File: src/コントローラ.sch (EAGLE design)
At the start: 13 parts, among them SW1 TOGGLESWITCH

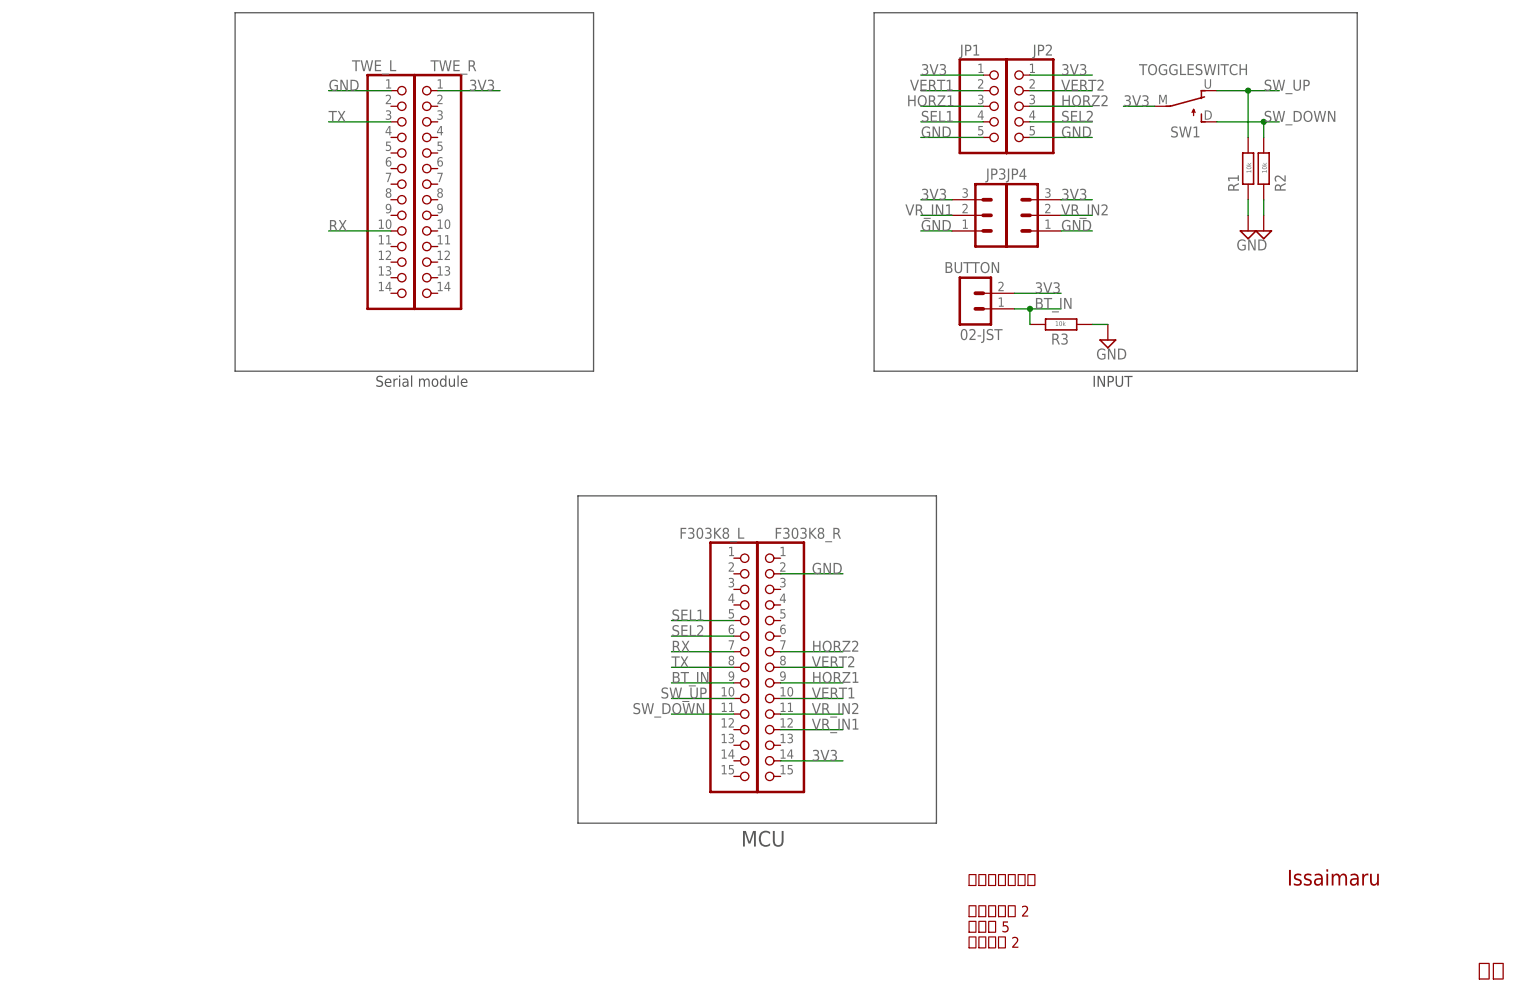
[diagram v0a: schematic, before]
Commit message: fix
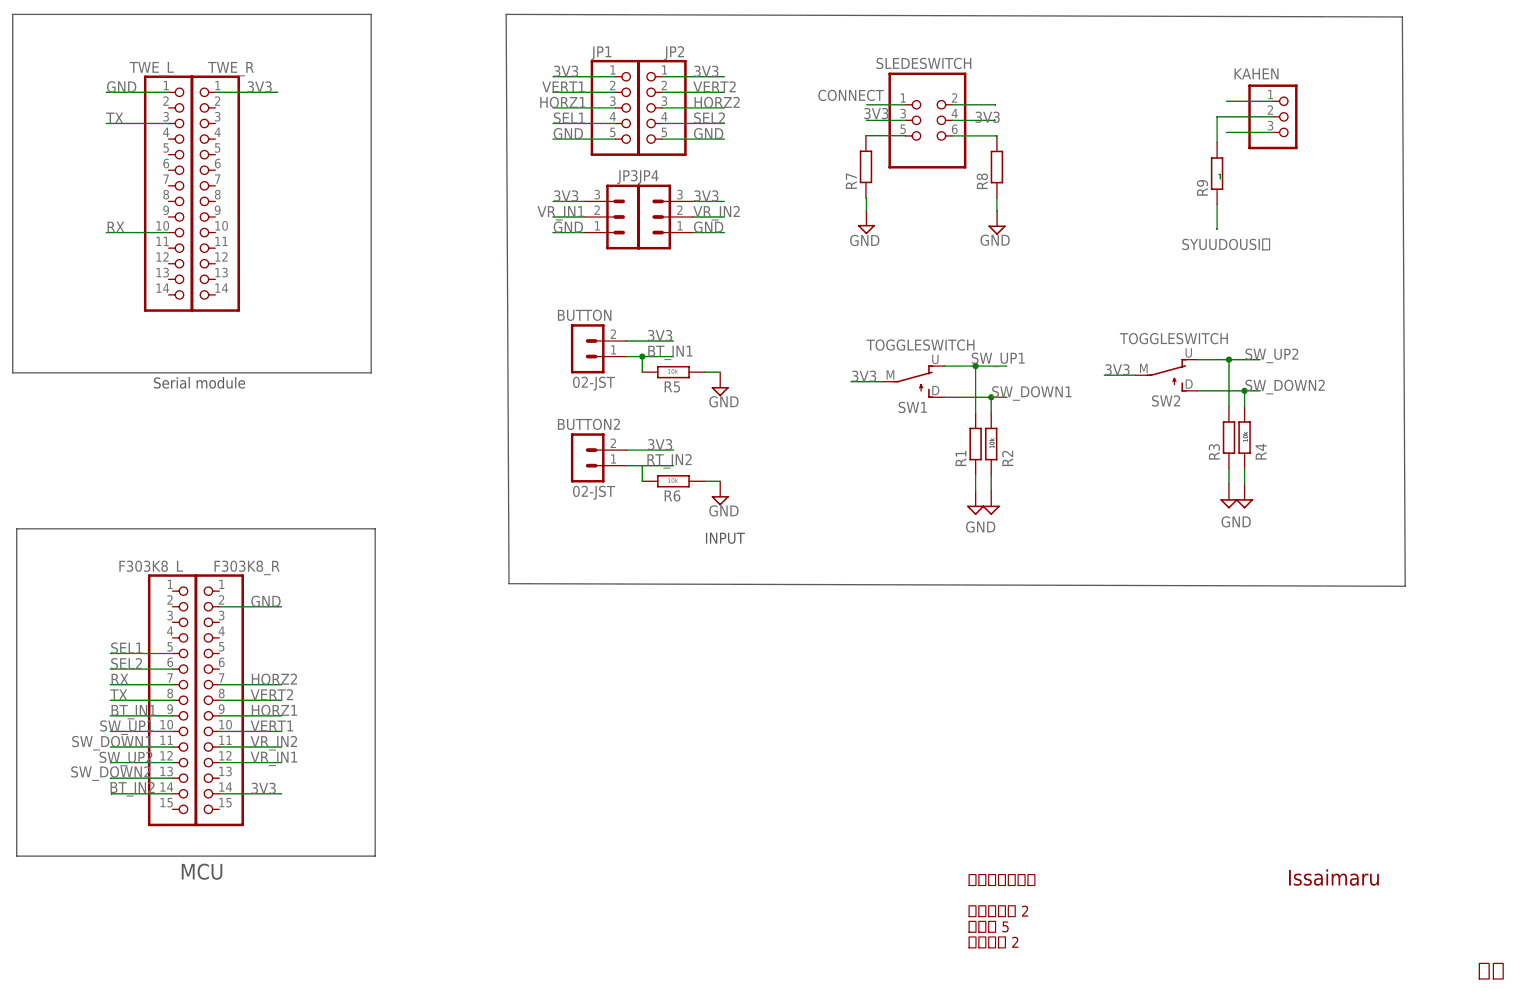
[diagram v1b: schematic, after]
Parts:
- added BUTTON2: 02-JST, con-jst-xh:02-JST
- added KAHEN: (no value), pinhead:PINHD-1X3
- added R4, R5, R6: 10k, rcl:R-EU_0204/7
- added R7, R8, R9: (no value), rcl:R-EU_0207/7
- added SLIDESWITCH: SLEDESWITCH, slide switch:SLEDESWITCH
- added SW2: TOGGLESWITCH, ToggleSwitch:TOGGLESWITCH
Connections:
- net SW_DOWN renamed SW_DOWN1
- net SW_UP renamed SW_UP1
- removed net BT_IN: BUTTON.1, F303K8_L.9, R3.2
- new net BT_IN1: BUTTON.1, F303K8_L.9, R5.2
- new net BT_IN2: F303K8_L.14, R6.2
- new net CONNECT: SLIDESWITCH.1
- new net CONNECT1: SLIDESWITCH.2
- new net N$1: R7.2, SLIDESWITCH.5
- new net N$2: R8.2, SLIDESWITCH.6
- new net N$5: KAHEN.2
- new net N$7: R9.1
- new net RT_IN2: BUTTON2.1
- new net SW_DOWN2: F303K8_L.13, R4.2, SW2.R
- new net SW_UP2: F303K8_L.12, R3.2, SW2.L
- new net SYUUDOUSI＋: R9.2
- net 3V3: now also BUTTON2.2, KAHEN.3, SLIDESWITCH.3, SLIDESWITCH.4, SW2.C
- net GND: now also KAHEN.1, R4.1, R5.1, R6.1, R7.1, R8.1
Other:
- note added: "GND"
- moved on the sheet: BUTTON, F303K8_L, F303K8_R, JP1, JP2, JP3, JP4, R1, R2, R3, SW1, TWE_L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
